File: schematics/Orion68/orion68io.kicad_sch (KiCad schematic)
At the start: 38 parts, among them J1 LevelConverter, J200 Euro96pin, U200 GAL16V8, U25 SN74LVC245APW, U26 SN74LVC245APW, U27 RP5C01A, U30 LM2937xT, Y3 Crystal

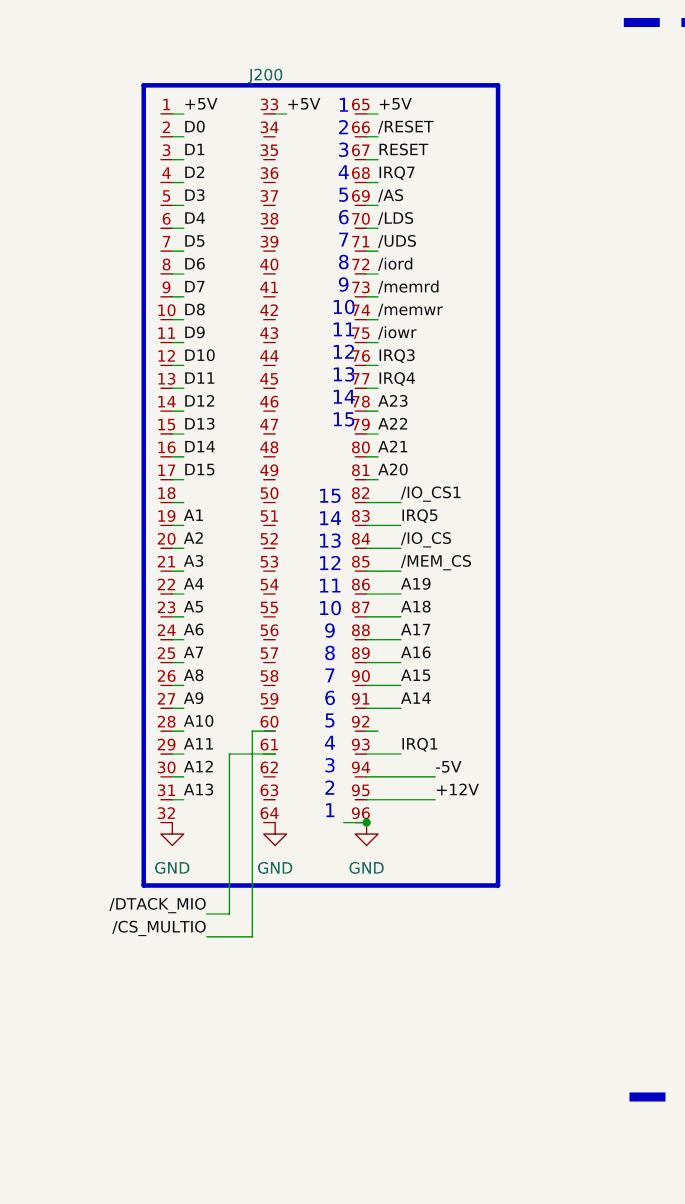
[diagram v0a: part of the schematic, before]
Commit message: Implemented new picoVGA V2
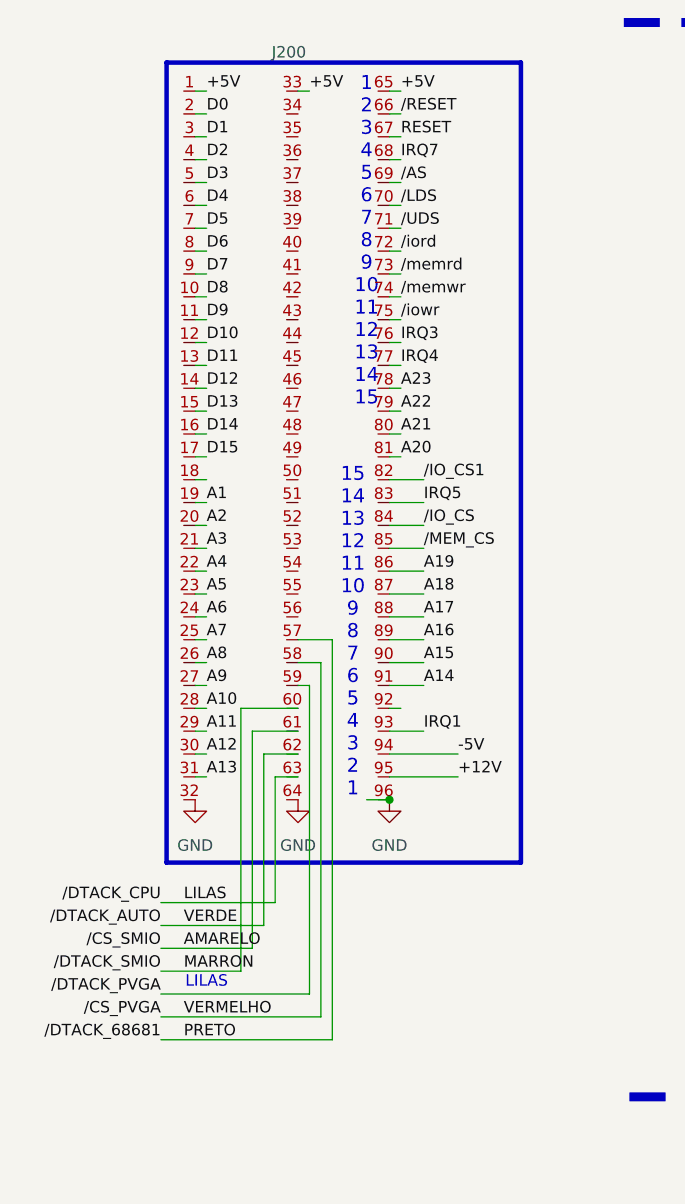
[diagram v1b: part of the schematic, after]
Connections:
- net /CS_MULTIO: no longer J200.60
- net /DTACK_MIO: no longer J200.61
- net PRETO: now reaches J200.57
- net VERMELHO: now reaches J200.58
- net /DTACK_PVGA: now reaches J200.59
- net VERDE: now reaches J200.62
- net LILAS: now reaches J200.63
- new net AMARELO: J200.61
- new net MARRON: J200.60
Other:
- note added: "LILAS"
